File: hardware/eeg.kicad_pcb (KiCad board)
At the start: 4 copper layers, 53.3 x 51.8 mm, 149 parts, among them IC1 TPS62162QDSGRQ1, IC10 INA333AIDRGT, IC11 OPA333AIDCKRG4, IC12 MCP602-E_SN, IC13 MCP602-E_SN, IC14 INA333AIDRGT, IC15 OPA333AIDCKRG4, IC16 MCP602-E_SN, IC17 MCP602-E_SN, IC18 INA333AIDRGT, IC19 OPA333AIDCKRG4, IC2 LT3042IMSE#PBF, IC20 MCP602-E_SN, IC21 MCP602-E_SN, IC22 OPA333AIDCKRG4, IC3 STM32H730VBT6, IC4 ESP32-C6-MINI-1-H4, IC5 W25Q512JVFIQ, IC6 INA333AIDRGT, IC7 OPA333AIDCKRG4, IC8 MCP602-E_SN, IC9 MCP602-E_SN, J1 Battery LiPO, J3 ST-Link, J4 Serial, J5 Serial, SW1 SW_Push_Dual, SW2 SW_Push_Dual, SW3 SW_Push_Dual, Y1 Crystal_GND24_Small, Y2 Crystal_GND24_Small

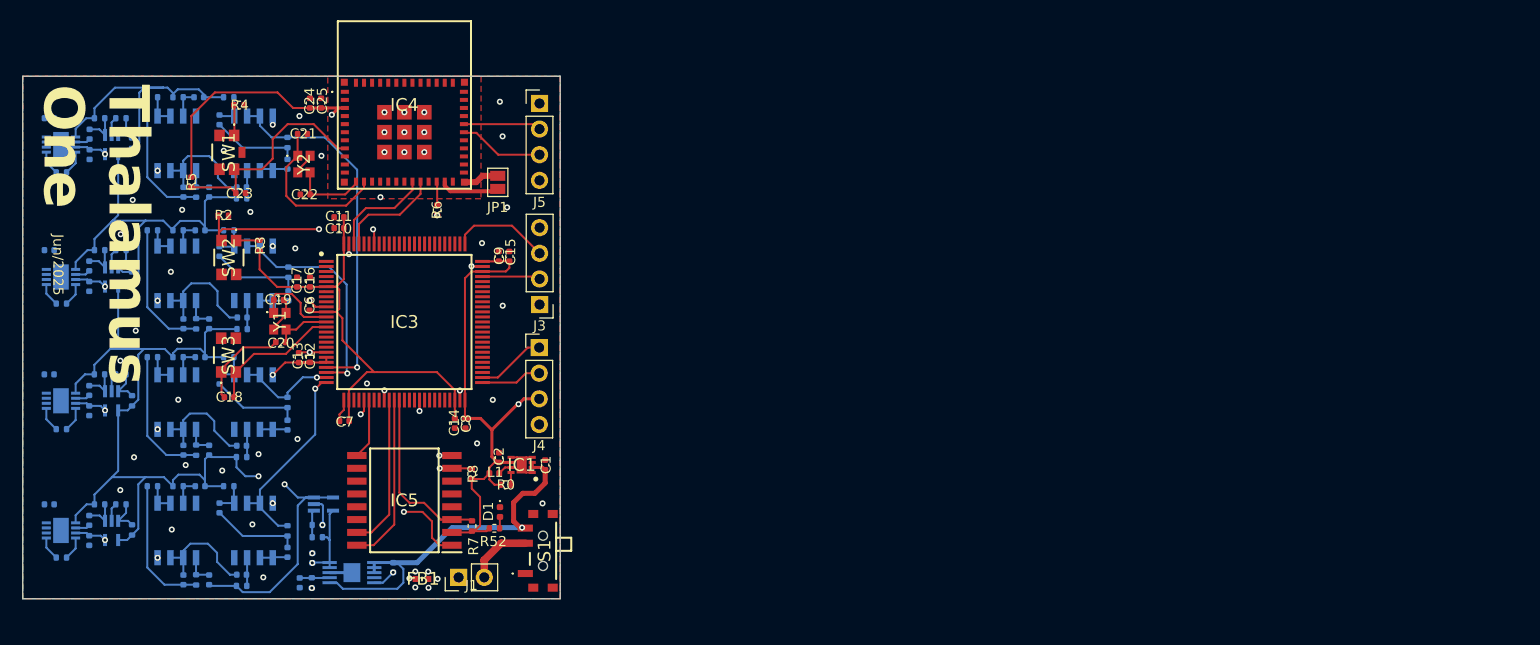
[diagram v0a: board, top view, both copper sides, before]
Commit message: hardware final update
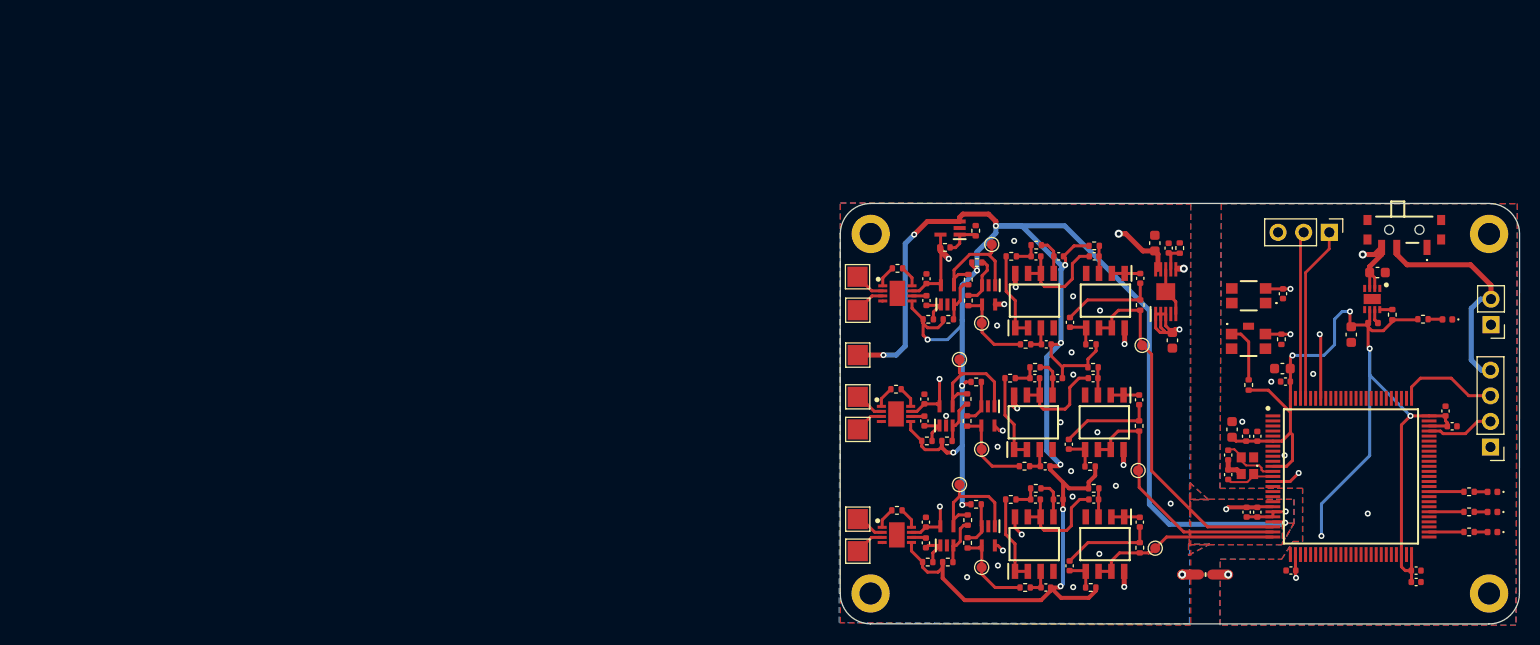
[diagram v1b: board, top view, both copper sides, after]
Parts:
- removed C45, C53, C54: 0.1uF, Capacitor_SMD:C_0402_1005Metric
- removed C46, C55: 330nF, Capacitor_SMD:C_0402_1005Metric
- removed C47, C48, C56, C57: 36nF, Capacitor_SMD:C_0402_1005Metric
- removed C49, C58: 8.2nF, Capacitor_SMD:C_0402_1005Metric
- removed C50, C51, C52, C59, C60, C61: 300nF, Capacitor_SMD:C_0402_1005Metric
- removed IC10, IC14, IC18, IC6: INA333AIDRGT, ina333:SON50P300X300X80-9N-D
- removed IC11, IC15, IC19, IC22, IC7: OPA333AIDCKRG4, opa333:SOT65P210X110-5N
- removed IC12, IC13, IC16, IC17, IC20, IC21, IC8, IC9: MCP602-E_SN, mcp602:SOIC127P600X175-8N
- removed IC5: W25Q512JVFIQ, w25q512jvfiq:SOIC127P1032X264-16N
- removed J5: Serial, Connector_PinHeader_2.54mm:PinHeader_1x04_P2.54mm_Vertical
- removed JP1: Jumper_2_Bridged, Jumper:SolderJumper-2_P1.3mm_Open_Pad1.0x1.5mm
- removed R0: 100k, Resistor_SMD:R_0402_1005Metric
- removed R47: 484k, Resistor_SMD:R_0402_1005Metric
- removed R48: 1.93M, Resistor_SMD:R_0402_1005Metric
- removed R50, R51: 10k, Resistor_SMD:R_0402_1005Metric
- removed R52: 1k, Resistor_SMD:R_0402_1005Metric
- removed SW1: SW_Push_Dual, tactile_button:TL1030AF160BQJ
- removed Y2: Crystal_GND24_Small, crystal30M:830107284409
- added CH1+: TestPoint, TestPoint:TestPoint_Pad_2.0x2.0mm, F.Cu at (144.5, 87.0)
- added CH1-: TestPoint, TestPoint:TestPoint_Pad_2.0x2.0mm, F.Cu at (144.5, 83.8)
- added CH2+: TestPoint, TestPoint:TestPoint_Pad_2.0x2.0mm, F.Cu at (144.5, 74.9)
- added CH2-: TestPoint, TestPoint:TestPoint_Pad_2.0x2.0mm, F.Cu at (144.5, 71.7)
- added CH3+: TestPoint, TestPoint:TestPoint_Pad_2.0x2.0mm, F.Cu at (144.5, 63.1)
- added CH3-: TestPoint, TestPoint:TestPoint_Pad_2.0x2.0mm, F.Cu at (144.5, 59.8)
- added D2: LED, LED_SMD:LED_0402_1005Metric, F.Cu at (207.4, 81.1)
- added D3: LED, LED_SMD:LED_0402_1005Metric, F.Cu at (207.4, 83.1)
- added D4: LED, LED_SMD:LED_0402_1005Metric, F.Cu at (207.4, 85.1)
- added G***: LOGO, logo:brain_2, B.Cu at (178.3, 71.7)
- added G***: LOGO, logo:st, B.Cu at (192.0, 91.1)
- added G***: LOGO, logo:logoUFU_2, B.Cu at (202.9, 91.0)
- added G***: LOGO, logo:logoFEELT_3, B.Cu at (199.0, 91.1)
- added G***: LOGO, logo:pinguim, B.Cu at (195.5, 91.1)
- added H1: MountingHole_Pad, MountingHole:MountingHole_2.2mm_M2_DIN965_Pad, F.Cu at (145.8, 55.6)
- added H2: MountingHole_Pad, MountingHole:MountingHole_2.2mm_M2_DIN965_Pad, F.Cu at (145.8, 91.2)
- added H3: MountingHole_Pad, MountingHole:MountingHole_2.2mm_M2_DIN965_Pad, F.Cu at (207.1, 55.6)
- added H4: MountingHole_Pad, MountingHole:MountingHole_2.2mm_M2_DIN965_Pad, F.Cu at (207.1, 91.2)
- added REF: TestPoint, TestPoint:TestPoint_Pad_2.0x2.0mm, F.Cu at (144.5, 67.6)
- added TP1: TestPoint, TestPoint:TestPoint_Pad_D1.0mm, F.Cu at (154.6, 80.4)
- added TP2: TestPoint, TestPoint:TestPoint_Pad_D1.0mm, F.Cu at (156.8, 88.6)
- added TP3: TestPoint, TestPoint:TestPoint_Pad_D1.0mm, F.Cu at (174.0, 86.7)
- added TP4: TestPoint, TestPoint:TestPoint_Pad_D1.0mm, F.Cu at (154.6, 68.0)
- added TP5: TestPoint, TestPoint:TestPoint_Pad_D1.0mm, F.Cu at (156.8, 76.9)
- added TP6: TestPoint, TestPoint:TestPoint_Pad_D1.0mm, F.Cu at (172.3, 79.0)
- added TP7: TestPoint, TestPoint:TestPoint_Pad_D1.0mm, F.Cu at (157.8, 56.6)
- added TP8: TestPoint, TestPoint:TestPoint_Pad_D1.0mm, F.Cu at (156.8, 64.4)
- added TP9: TestPoint, TestPoint:TestPoint_Pad_D1.0mm, F.Cu at (172.7, 66.6)
- added U1: INA333xxDRG, ina333:SON50P300X300X80-9N-D, F.Cu at (148.4, 85.4)
- added U10: OPA333xxDCK, opa333:SOT65P210X110-5N, F.Cu at (153.4, 61.6)
- added U11: MCP602, mcp602:SOIC127P600X175-8N, F.Cu at (162.0, 62.2)
- added U12: MCP602, mcp602:SOIC127P600X175-8N, F.Cu at (169.1, 62.2)
- added U17: OPA333xxDCK, opa333:SOT65P210X110-5N, F.Cu at (157.5, 85.5)
- added U18: OPA333xxDCK, opa333:SOT65P210X110-5N, F.Cu at (157.4, 73.6)
- added U19: OPA333xxDCK, opa333:SOT65P210X110-5N, F.Cu at (157.5, 61.6)
- added U2: OPA333xxDCK, opa333:SOT65P210X110-5N, F.Cu at (153.4, 85.5)
- added U3: MCP602, mcp602:SOIC127P600X175-8N, F.Cu at (162.0, 86.3)
- added U4: MCP602, mcp602:SOIC127P600X175-8N, F.Cu at (169.0, 86.3)
- added U5: INA333xxDRG, ina333:SON50P300X300X80-9N-D, F.Cu at (148.3, 73.4)
- added U6: OPA333xxDCK, opa333:SOT65P210X110-5N, F.Cu at (153.3, 73.6)
- added U7: MCP602, mcp602:SOIC127P600X175-8N, F.Cu at (161.9, 74.2)
- added U8: MCP602, mcp602:SOIC127P600X175-8N, F.Cu at (169.0, 74.2)
- added U9: INA333xxDRG, ina333:SON50P300X300X80-9N-D, F.Cu at (148.5, 61.5)
- C1: value 10uF -> 0.1uF
- C10: value 100nF -> 330nF
- C11: value 10uF -> 36nF
- C12: value 100nF -> 8.2nF
- C13: value 1uF -> 36nF
- C14, C15: value 2.2uF -> 300nF
- C16, C6, C7, C8: value 100nF -> 300nF
- C17: value 4.7uF -> 0.1uF
- C18: value 0.1uF -> 330nF
- C19, C21: value 20pF -> 36nF
- C2: value 22uF -> 330nF
- C20: value 20pF -> 8.2nF
- C22: value 20pF -> 300nF
- C23: value 1uF -> 300nF
- C24: value 22uF -> 300nF
- C25: value 0.1uF -> 100nF
- C26, C27, C35: value 0.1uF -> 100nF; moved to F.Cu
- C28: value 330nF -> 100nF; moved to F.Cu
- C29: value 36nF -> 100nF; moved to F.Cu
- C3, C5: value 4.7uF -> 36nF; moved to F.Cu
- C30: value 36nF -> 10uF; footprint Capacitor_SMD:C_0402_1005Metric -> Capacitor_SMD:C_0603_1608Metric; moved to F.Cu
- C31: value 8.2nF -> 100nF; moved to F.Cu
- C32: value 300nF -> 1uF; moved to F.Cu
- C33, C34: value 300nF -> 2.2uF; moved to F.Cu
- C36: value 0.1uF -> 4.7uF; footprint Capacitor_SMD:C_0402_1005Metric -> Capacitor_SMD:C_0603_1608Metric; moved to F.Cu
- C37: value 330nF -> 20pF; moved to F.Cu
- C38: value 36nF -> 20pF; moved to F.Cu
- C39: value 36nF -> 0.1uF; moved to F.Cu
- C4: value 0.47uF -> 8.2nF; moved to F.Cu
- C40: value 8.2nF -> 4.7uF; footprint Capacitor_SMD:C_0402_1005Metric -> Capacitor_SMD:C_0603_1608Metric; moved to F.Cu
- C41: value 300nF -> 0.47uF; moved to F.Cu
- C42: value 300nF -> 4.7uF; footprint Capacitor_SMD:C_0402_1005Metric -> Capacitor_SMD:C_0603_1608Metric; moved to F.Cu
- C43: value 300nF -> 10uF; footprint Capacitor_SMD:C_0402_1005Metric -> Capacitor_SMD:C_0603_1608Metric; moved to F.Cu
- C44: value 0.1uF -> 22uF; footprint Capacitor_SMD:C_0402_1005Metric -> Capacitor_SMD:C_0603_1608Metric; moved to F.Cu
- C9: value 100nF -> 0.1uF
- IC2, R31, R32, R33, R34, R35, R36: moved to F.Cu
- IC4: value ESP32-C6-MINI-1-H4 -> OPA333AIDCKRG4; footprint esp32c6:ESP32C6MINI1H4 -> opa333:SOT65P210X110-5N
- J4: footprint Connector_PinHeader_2.54mm:PinHeader_1x04_P2.54mm_Vertical -> Connector_PinHeader_2.54mm:PinHeader_1x03_P2.54mm_Vertical
- R1: value 33.2k -> 10k; moved to F.Cu
- R10: value 910k -> 149K; moved to F.Cu
- R11: value 1.5k -> 276K; moved to F.Cu
- R12: value 750k -> 967k; moved to F.Cu
- R13: value 97k -> 1.93M; moved to F.Cu
- R14: value 149K -> 484k; moved to F.Cu
- R15: value 276K -> 5.26k; moved to F.Cu
- R16: value 967k -> 910k; moved to F.Cu
- R17: value 484k -> 1.5k; moved to F.Cu
- R18: value 1.93M -> 750k; moved to F.Cu
- R19, R29: value 5.26k -> 1.5k; moved to F.Cu
- R20, R30: value 910k -> 750k; moved to F.Cu
- R21: value 1.5k -> 97k; moved to F.Cu
- R22: value 750k -> 149K; moved to F.Cu
- R23: value 97k -> 276K; moved to F.Cu
- R24: value 149K -> 967k; moved to F.Cu
- R25: value 276K -> 1.93M; moved to F.Cu
- R26: value 967k -> 484k; moved to F.Cu
- R27: value 484k -> 5.26k; moved to F.Cu
- R28: value 1.93M -> 910k; moved to F.Cu
- R3: value 1k -> 5.26k
- R37: value 484k -> 1.93M; moved to F.Cu
- R38: value 1.93M -> 484k; moved to F.Cu
- R39: value 5.26k -> 1k; moved to F.Cu
- R4: value 1k -> 910k
- R40: value 910k -> 1k; moved to F.Cu
- R41: value 1.5k -> 1k; moved to F.Cu
- R42: value 750k -> 1k; moved to F.Cu
- R43: value 97k -> 10k; moved to F.Cu
- R44: value 149K -> 1k; moved to F.Cu
- R45: value 276K -> 33.2k; moved to F.Cu
- R46: value 967k -> 100k; moved to F.Cu
- R5, R7: value 10k -> 1.5k
- R6, R8: value 10k -> 750k
- R9: value 5.26k -> 97k; moved to F.Cu
- SW2: footprint tactile_button:TL1030AF200AQJ -> tactile_button:TL1030AF160BQJ
- moved R39 143.0 mm to (205.1, 81.1)
- moved R40 141.2 mm to (205.1, 83.1), turned to 0 degrees
- moved R41 139.7 mm to (205.1, 85.1)
- moved C28 134.8 mm to (202.8, 73.1)
- moved C27 131.5 mm to (199.8, 88.9), turned to 0 degrees
- moved C44 129.3 mm to (193.4, 65.5), turned to -90 degrees
- moved R44 127.8 mm to (200.5, 64.0)
- moved C26 123.2 mm to (187.4, 88.9)
- moved C34 122.4 mm to (203.4, 74.6), turned to 0 degrees
- moved C35 119.9 mm to (184.1, 75.6), turned to 90 degrees
- moved C43 115.2 mm to (196.0, 59.4), turned to 0 degrees
- moved R46 114.6 mm to (197.5, 63.6), turned to -90 degrees
- moved C36 113.3 mm to (181.6, 74.9), turned to 90 degrees
- moved R42 113.2 mm to (183.3, 70.5), turned to -90 degrees
- moved C37 113.0 mm to (181.2, 77.5), turned to -90 degrees
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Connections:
- C1 pad 1: VIN_BAT -> GNDA
- C1 pad 2: GND -> VDDA33
- C10 pad 1: VBAT -> Net-(C10-Pad1)
- C10 pad 2: GND -> Net-(U6-+)
- C11 pad 1: VBAT -> Net-(U7A-+)
- C11 pad 2: GND -> VREF
- C12 pad 1: VDDA33 -> Net-(U7B-+)
- C12 pad 2: GNDA -> VREF
- C13 pad 1: VDDA33 -> Net-(C13-Pad1)
- C13 pad 2: GNDA -> Net-(U7B--)
- C14 pad 1: VBAT -> Net-(U8A-+)
- C14 pad 2: GND -> Net-(U7B--)
- C15 pad 1: VBAT -> Net-(C15-Pad1)
- C15 pad 2: GND -> Net-(U8A--)
- C16 pad 1: VBAT -> Net-(U8B-+)
- C16 pad 2: GND -> Net-(C15-Pad1)
- C17 pad 1: VBAT -> GNDA
- C17 pad 2: GND -> VDDA33
- C18 pad 1: RESET -> Net-(C18-Pad1)
- C18 pad 2: GND -> Net-(U10-+)
- C19 pad 1: HSE_I -> Net-(U11A-+)
- C19 pad 2: GND -> VREF
- C2 pad 1: VBAT -> Net-(C2-Pad1)
- C2 pad 2: GND -> Net-(U2-+)
- C20 pad 1: HSE_O -> Net-(U11B-+)
- C20 pad 2: GND -> VREF
- C21 pad 1: XTAL_32K_P -> Net-(C21-Pad1)
- C21 pad 2: GND -> Net-(U11B--)
- C22 pad 1: XTAL_32K_N -> Net-(U12A-+)
- C22 pad 2: GND -> Net-(U11B--)
- C23 pad 1: ESP-RESET -> Net-(C23-Pad1)
- C23 pad 2: GND -> Net-(U12A--)
- C24 pad 1: VBAT -> Net-(U12B-+)
- C24 pad 2: GND -> Net-(C23-Pad1)
- C26 pad 1: GNDA -> VBAT
- C26 pad 2: GNDA -> GND
- C27 pad 1: VDDA33 -> VBAT
- C27 pad 2: GNDA -> GND
- C28 pad 1: Net-(IC6-VOUT) -> VBAT
- C28 pad 2: LNA_OUT_0 -> GND
- C29 pad 1: BPF_V+_STG0_0 -> VBAT
- C29 pad 2: PGA_OUT_0 -> GND
- C3 pad 1: VIN_BAT -> Net-(U3A-+)
- C3 pad 2: GNDA -> VREF
- C30 pad 1: Net-(C30-Pad1) -> VBAT
- C30 pad 2: BPF_V-_STG1_0 -> GND
- C31 pad 1: BPF_V+_STG1_0 -> VDDA33
- C31 pad 2: PGA_OUT_0 -> GNDA
- C32 pad 1: BPF_V+_STG2_0 -> VDDA33
- C32 pad 2: BPF_V-_STG1_0 -> GNDA
- C33 pad 1: Net-(C33-Pad1) -> VBAT
- C33 pad 2: BPF_V-_STG2_0 -> GND
- C34 pad 1: BPF_V+_STG3_0 -> VBAT
- C34 pad 2: Net-(C33-Pad1) -> GND
- C35 pad 1: GNDA -> VBAT
- C35 pad 2: GNDA -> GND
- C36 pad 1: VDDA33 -> VBAT
- C36 pad 2: GNDA -> GND
- C37 pad 1: Net-(IC10-VOUT) -> HSE_I
- C37 pad 2: LNA_OUT_1 -> GND
- C38 pad 1: BPF_V+_STG0_1 -> HSE_O
- C38 pad 2: PGA_OUT_0 -> GND
- C39 pad 1: Net-(C39-Pad1) -> RESET
- C39 pad 2: BPF_V-_STG1_1 -> GND
- C4 pad 1: Net-(IC2-SET) -> Net-(U3B-+)
- C4 pad 2: GNDA -> VREF
- C40 pad 1: BPF_V+_STG1_1 -> VIN_BAT
- C40 pad 2: PGA_OUT_0 -> GNDA
- C41 pad 1: BPF_V+_STG2_1 -> Net-(IC2-SET)
- C41 pad 2: BPF_V-_STG1_1 -> GNDA
- C42 pad 1: Net-(C42-Pad1) -> VDDA33
- C42 pad 2: BPF_V-_STG2_1 -> GNDA
- C43 pad 1: BPF_V+_STG3_1 -> VIN_BAT
- C43 pad 2: Net-(C42-Pad1) -> GND
- C44 pad 1: GNDA -> VBAT
- C44 pad 2: GNDA -> GND
- C5 pad 1: VDDA33 -> Net-(C5-Pad1)
- C5 pad 2: GNDA -> Net-(U3B--)
- C6 pad 1: VBAT -> Net-(U4A-+)
- C6 pad 2: GND -> Net-(U3B--)
- C7 pad 1: VBAT -> Net-(C7-Pad1)
- C7 pad 2: GND -> Net-(U4A--)
- C8 pad 1: VBAT -> Net-(U4B-+)
- C8 pad 2: GND -> Net-(C7-Pad1)
- C9 pad 1: VBAT -> GNDA
- C9 pad 2: GND -> VDDA33
- IC3 pad 15: unconnected-(IC3-PC0-Pad15) -> GND
- IC3 pad 18: unconnected-(IC3-PC3_C-Pad18) -> GNDA
- IC3 pad 22: ADC_IN3 -> VREF
- IC3 pad 23: ADC_IN2 -> ADC_IN3
- IC3 pad 24: ADC_IN1 -> ADC_IN2
- IC3 pad 25: ADC_IN0 -> ADC_IN1
- IC3 pad 51: UART5_RX -> unconnected-(IC3-PB12-Pad51)
- IC3 pad 52: UART5_TX -> LED_3
- IC3 pad 56: unconnected-(IC3-PD9-Pad56) -> LED_2
- IC3 pad 60: unconnected-(IC3-PD13-Pad60) -> LED_1
- IC3 pad 69: USB_OTG_HS_ID -> unconnected-(IC3-PA10-Pad69)
- IC3 pad 70: USB_OTG_HS_DM -> unconnected-(IC3-PA11-Pad70)
- IC3 pad 71: USB_OTG_HS_DP -> unconnected-(IC3-PA12-Pad71)
- IC4 pad 1: GND -> Net-(IC4-+IN)
- IC4 pad 2: GND -> GNDA
- IC4 pad 3: VBAT -> VREF
- IC4 pad 4: unconnected-(IC4-NC_1-Pad4) -> VREF
- IC4 pad 5: unconnected-(IC4-IO2-Pad5) -> VDDA33
- J1 pad 2: Net-(J1-Pin_2) -> VIN_SWT
- J3 pad 1: VBAT -> GND
- J3 pad 4: GND -> VIN_SWT
- J4 pad 1: UART5_TX -> MCU_RX
- J4 pad 2: UART5_RX -> MCU_TX
- J4 pad 3: VBAT -> GND
- R1 pad 1: Net-(IC2-SET) -> Net-(IC4-+IN)
- R1 pad 2: GNDA -> VDDA33
- R10 pad 1: LNA_OUT_0 -> Net-(C5-Pad1)
- R10 pad 2: PGA_OUT_0 -> Net-(U3A--)
- R11 pad 1: GNDA -> Net-(C5-Pad1)
- R11 pad 2: Net-(IC7--IN) -> Net-(U3B-+)
- R12 pad 1: PGA_OUT_0 -> VREF
- R12 pad 2: Net-(IC7--IN) -> Net-(U4A-+)
- R13 pad 1: PGA_OUT_0 -> VREF
- R13 pad 2: BPF_V+_STG0_0 -> Net-(U4B-+)
- R14 pad 1: Net-(C30-Pad1) -> ADC_IN1
- R14 pad 2: BPF_V-_STG0_0 -> Net-(C7-Pad1)
- R15 pad 1: Net-(C30-Pad1) -> Net-(R15-Pad1)
- R15 pad 2: BPF_V+_STG1_0 -> Net-(R15-Pad2)
- R16 pad 1: PGA_OUT_0 -> Net-(U6-+)
- R16 pad 2: BPF_V+_STG2_0 -> VREF
- R17 pad 1: ADC_IN0 -> Net-(U6--)
- R17 pad 2: Net-(C33-Pad1) -> VREF
- R18 pad 1: PGA_OUT_0 -> Net-(U6--)
- R18 pad 2: BPF_V+_STG3_0 -> Net-(U18-+)
- R19 pad 1: Net-(IC10-RG_1) -> Net-(U18--)
- R19 pad 2: Net-(IC10-RG_2) -> VREF
- R2 pad 1: GND -> GNDA
- R2 pad 2: BOOT -> Net-(IC4-+IN)
- R20 pad 1: LNA_OUT_1 -> Net-(U18--)
- R20 pad 2: PGA_OUT_0 -> Net-(R20-Pad2)
- R21 pad 1: GNDA -> Net-(R20-Pad2)
- R21 pad 2: Net-(IC11--IN) -> Net-(U7A-+)
- R22 pad 1: PGA_OUT_0 -> Net-(C13-Pad1)
- R22 pad 2: Net-(IC11--IN) -> Net-(U7A--)
- R23 pad 1: PGA_OUT_0 -> Net-(C13-Pad1)
- R23 pad 2: BPF_V+_STG0_1 -> Net-(U7B-+)
- R24 pad 1: Net-(C39-Pad1) -> VREF
- R24 pad 2: BPF_V-_STG0_1 -> Net-(U8A-+)
- R25 pad 1: Net-(C39-Pad1) -> VREF
- R25 pad 2: BPF_V+_STG1_1 -> Net-(U8B-+)
- R26 pad 1: PGA_OUT_0 -> ADC_IN2
- R26 pad 2: BPF_V+_STG2_1 -> Net-(C15-Pad1)
- R27 pad 1: ADC_IN1 -> Net-(R27-Pad1)
- R27 pad 2: Net-(C42-Pad1) -> Net-(R27-Pad2)
- R28 pad 1: PGA_OUT_0 -> Net-(U10-+)
- R28 pad 2: BPF_V+_STG3_1 -> VREF
- R29 pad 1: Net-(IC14-RG_1) -> Net-(U10--)
- R29 pad 2: Net-(IC14-RG_2) -> VREF
- R3 pad 2: VBAT -> Net-(R3-Pad2)
- R30 pad 1: LNA_OUT_2 -> Net-(U10--)
- R30 pad 2: PGA_OUT_0 -> Net-(U19-+)
- R31 pad 1: GNDA -> Net-(U19--)
- R31 pad 2: Net-(IC15--IN) -> VREF
- R32 pad 1: PGA_OUT_0 -> Net-(U19--)
- R32 pad 2: Net-(IC15--IN) -> Net-(R32-Pad2)
- R33 pad 1: PGA_OUT_0 -> Net-(R32-Pad2)
- R33 pad 2: BPF_V+_STG0_2 -> Net-(U11A-+)
- R34 pad 1: Net-(C48-Pad1) -> Net-(C21-Pad1)
- R34 pad 2: BPF_V-_STG0_2 -> Net-(U11A--)
- R35 pad 1: Net-(C48-Pad1) -> Net-(C21-Pad1)
- R35 pad 2: BPF_V+_STG1_2 -> Net-(U11B-+)
- R36 pad 1: PGA_OUT_0 -> VREF
- R36 pad 2: BPF_V+_STG2_2 -> Net-(U12A-+)
- R37 pad 1: ADC_IN2 -> VREF
- R37 pad 2: Net-(C51-Pad1) -> Net-(U12B-+)
- R38 pad 1: PGA_OUT_0 -> ADC_IN3
- R38 pad 2: BPF_V+_STG3_2 -> Net-(C23-Pad1)
- R39 pad 1: Net-(IC18-RG_1) -> LED_1
- R4 pad 1: Net-(R4-Pad1) -> Net-(U2-+)
- R4 pad 2: GND -> VREF
- R40 pad 1: LNA_OUT_3 -> LED_2
- R40 pad 2: PGA_OUT_0 -> Net-(D3-A)
- R41 pad 1: GNDA -> LED_3
- R41 pad 2: Net-(IC19--IN) -> Net-(D4-A)
- R42 pad 1: PGA_OUT_0 -> Net-(R42-Pad1)
- R42 pad 2: Net-(IC19--IN) -> VBAT
- R43 pad 1: PGA_OUT_0 -> GND
- R43 pad 2: BPF_V+_STG0_3 -> BOOT
- R44 pad 1: Net-(C57-Pad1) -> VBAT
- R44 pad 2: BPF_V-_STG0_3 -> Net-(D1-A)
- R45 pad 1: Net-(C57-Pad1) -> Net-(IC2-SET)
- R45 pad 2: BPF_V+_STG1_3 -> GNDA
- R46 pad 1: PGA_OUT_0 -> Net-(IC1-PG)
- R46 pad 2: BPF_V+_STG2_3 -> VBAT
- R5 pad 1: VBAT -> Net-(U2--)
- R5 pad 2: ESP-RESET -> VREF
- R6 pad 1: VBAT -> Net-(U2--)
- R6 pad 2: Net-(IC4-IO8) -> Net-(U17-+)
- R7 pad 1: RESET_FLASH -> Net-(U17--)
- R7 pad 2: VBAT -> VREF
- R8 pad 1: QSPI_NCS -> Net-(U17--)
- R8 pad 2: VBAT -> Net-(R8-Pad2)
- R9 pad 1: Net-(IC6-RG_1) -> Net-(R8-Pad2)
- R9 pad 2: Net-(IC6-RG_2) -> Net-(U3A-+)
- S1 pad 2: Net-(J1-Pin_2) -> VIN_SWT
- SW2 pad 1: Net-(R3-Pad1) -> Net-(R42-Pad1)
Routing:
- net VREF: track 0.00 -> 221.6 mm, vias 0 -> 14
- net PGA_OUT_0: track 179.3 -> 0.00 mm, vias 2 -> 0
- net VBAT: track 184.4 -> 108.5 mm, vias 3 -> 6
- net VDDA33: track 153.5 -> 184.9 mm, vias 13 -> 14
- net GND: track 31.4 -> 4.70 mm, vias 29 -> 6
- net QSPI_IO3: track 24.8 -> 0.00 mm, vias 2 -> 0
- net VIN_SWT: track 0.00 -> 22.5 mm
- net ESP-RESET: track 22.0 -> 0.00 mm
- net ADC_IN0: track 20.1 -> 0.00 mm, vias 1 -> 0
- net RESET_FLASH: track 17.1 -> 0.00 mm
- net QSPI_CLK: track 16.9 -> 0.00 mm
- net XTAL_32K_P: track 16.1 -> 0.00 mm
- net QSPI_IO0: track 14.9 -> 0.00 mm
- net RESET: track 13.4 -> 28.0 mm, vias 0 -> 2
- net QSPI_IO1: track 13.7 -> 0.00 mm, vias 2 -> 0
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- added copper zone on B.Cu, net GND
- added copper zone on In2.Cu, net GND
- added copper zone on F.Cu, net GNDA
- added copper zone on In1.Cu, net GNDA
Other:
- board size 53.3 x 51.8 mm -> 67.3 x 41.7 mm
- board text added: "Stephan C. Barros Heitor P. Cunha Enzo F. Rodrigues Ana Luiza I. Rosa Bernardo C. Trindade"
- board text added: "ThalamusOne"
- board text removed: "Jun/2025"
- board text removed: "Thalamus One"
